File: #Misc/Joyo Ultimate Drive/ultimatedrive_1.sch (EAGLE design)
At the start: 36 parts, among them Q1 MSPA18, U2 JRC4558D, U3 NE5532N

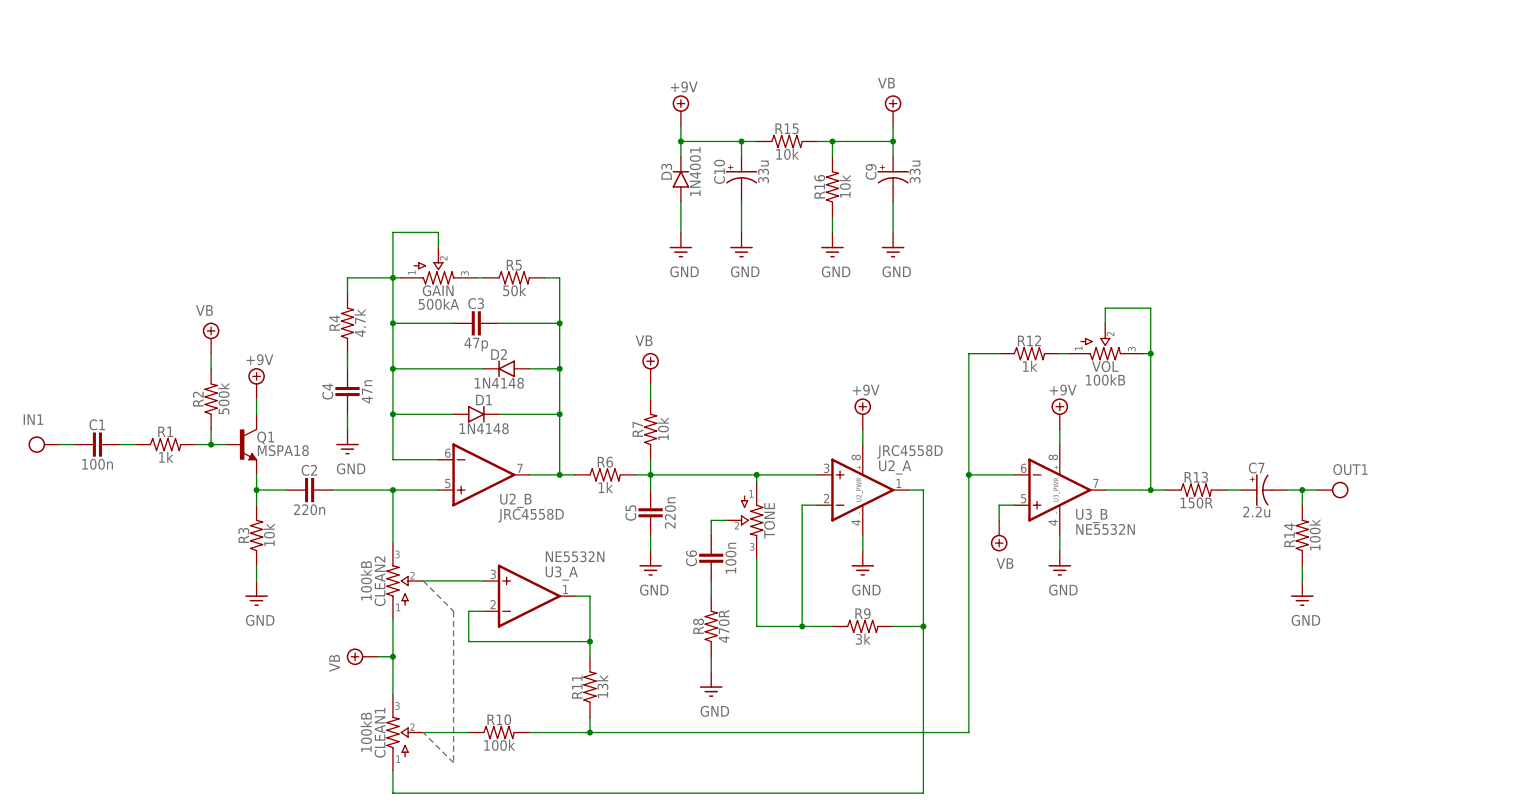
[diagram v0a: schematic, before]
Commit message: 20200320/09:17
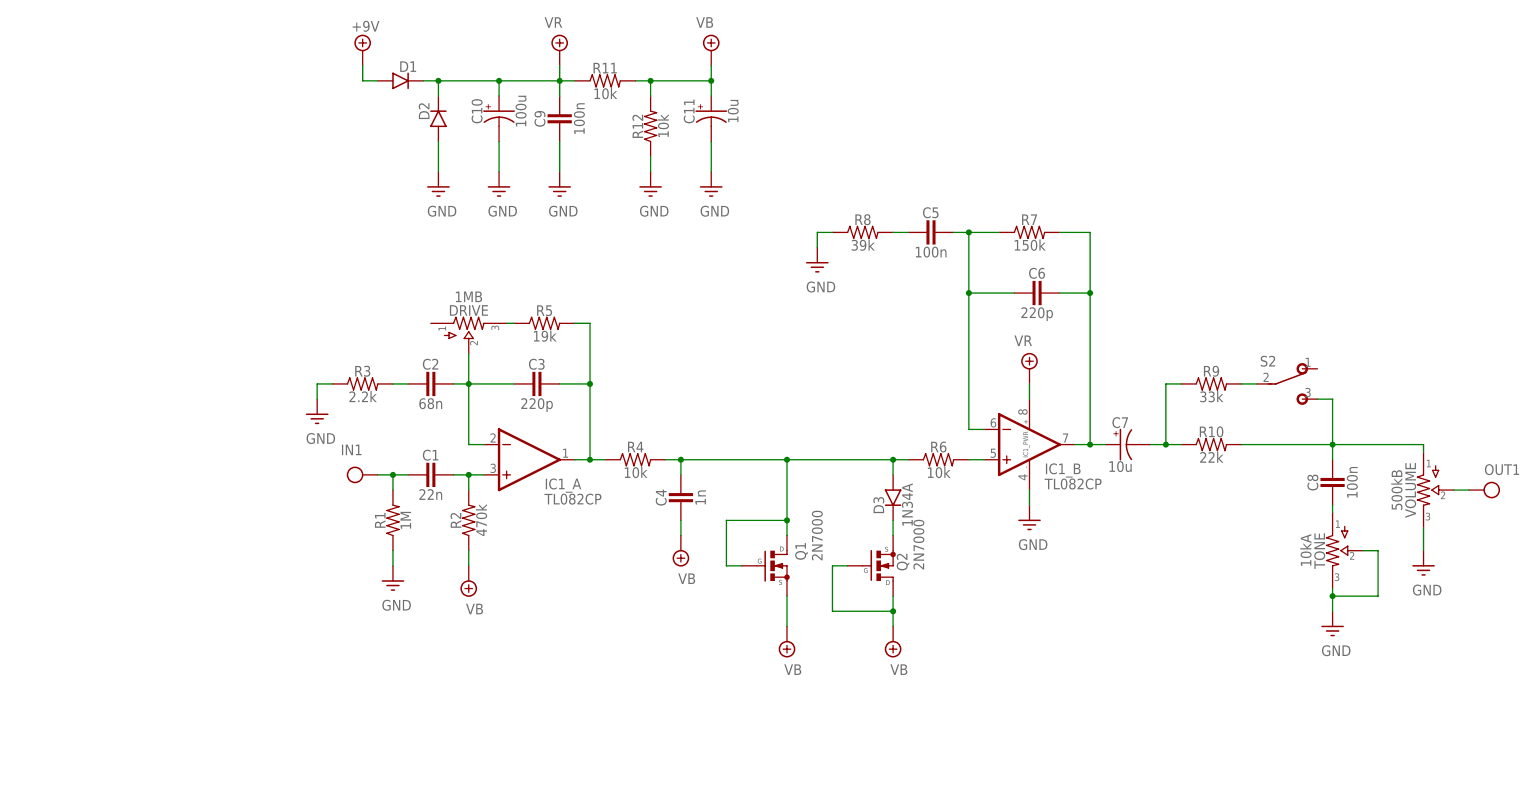
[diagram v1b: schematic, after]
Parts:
- removed CLEAN1, CLEAN2, VOL: 100kB, pedals-potentiometers:POTS16MM
- removed GAIN: 500kA, pedals-potentiometers:POTS16MM
- removed R13: 150R, pedals-resistors:R_.3B
- removed R14: 100k, pedals-resistors:R_.3B
- removed R15, R16: 10k, pedals-resistors:R_.3B
- removed U2: JRC4558D, pedals-integrated circuits:DUALTH
- removed U3: NE5532N, pedals-integrated circuits:DUALTH
- added C11: 10u, pedals-capacitors-elec:0500
- added C8: 100n, pedals-capacitors-film:CER/FILMBOX.1
- added DRIVE: 1MB, pedals-potentiometers:POTS16MM
- added IC1: TL082CP, pedals-integrated circuits:DUALTH
- added Q2: 2N7000, pedals-transistors:2N7000
- added S2: (no value), pedals-switches:SPDT
- added VOLUME: 500kB, pedals-potentiometers:POTS16MM
- C1: value 100n -> 22n
- C10: value 33u -> 100u
- C2: value 220n -> 68n
- C3: value 47p -> 220p
- C4: value 47n -> 1n
- C5: value 220n -> 100n
- C6: value 100n -> 220p
- C7: value 2.2u -> 10u
- C9: value 33u -> 100n; device pedals-capacitors-elec:0500 -> pedals-capacitors-film:CER/FILMBOX.1
- D1, D2: value 1N4148 -> (none); device pedals-diodes:DO35.2 -> pedals-diodes:DO41.3
- D3: value 1N4001 -> 1N34A; device pedals-diodes:DO35.3 -> pedals-diodes:DO41.2
- Q1: value MSPA18 -> 2N7000; device pedals-transistors:2N3904 -> pedals-transistors:2N7000
- R1: value 1k -> 1M
- R10: value 100k -> 22k
- R11: value 13k -> 10k
- R12, R6: value 1k -> 10k
- R2: value 500k -> 470k
- R3: value 10k -> 2.2k
- R4: value 4.7k -> 10k
- R5: value 50k -> 19k
- R7: value 10k -> 150k
- R8: value 470R -> 39k
- R9: value 3k -> 33k
- TONE: value (none) -> 10kA
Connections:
- removed net N$17: CLEAN1.1, R9.2, U2_A.OUT
- removed net N$18: CLEAN2.2, U3_A.+IN
- removed net N$19: C5.1, R6.2, R7.1, TONE.1, U2_A.+IN
- removed net N$21: C6.1, TONE.2
- removed net N$22: C6.2, R8.2
- removed net N$24: R12.2, VOL.1
- removed net N$25: R13.1, U3_B.OUT, VOL.2, VOL.3
- removed net N$28: C7.+, R13.2
- removed net N$3: GAIN.3, R5.1
- new net N$10: D3.C, Q2.S
- new net N$11: C4.1, D3.A, Q1.D, Q1.G, R4.2, R6.1
- new net N$16: C8.1, R10.2, S2.S, VOLUME.1
- new net N$7: C3.1, IC1_A.OUT, R4.1, R5.2
- new net VR: C10.+, C9.1, D1.C, D2.C, IC1_PWR.V+, R11.1
- net +9V: now also D1.A; no longer C10.+, D3.C, Q1.C, R15.1, U2_PWR.V+, U3_PWR.V+
- net GND: now also C11.-, C9.2, D2.A, IC1_PWR.V-, R1.1, R12.1, TONE.2, TONE.3, VOLUME.3; no longer C4.2, C5.2, C9.-, D3.A, R14.1, R16.1, U2_PWR.V-, U3_PWR.V-
- net IN: now also R1.2
- net N$1: now also C7.-, R10.1, R9.1; no longer C3.2, D1.A, D2.C, GAIN.1, GAIN.2, R4.2, U2_B.-IN
- net N$12: now also C5.1, C6.2, IC1_B.-IN, R7.1; no longer CLEAN1.2, R10.1
- net N$13: now also C6.1, C7.+, IC1_B.OUT, R7.2; no longer R11.2, U3_A.-IN, U3_A.OUT
- net N$14: now also C5.2, R8.2; no longer R9.1, TONE.3, U2_A.-IN
- net N$15: now also R9.2, S2.P; no longer R10.2, R11.1, R12.1, U3_B.-IN
- net N$2: now also C8.2, TONE.1; no longer C4.1, R4.1
- net N$4: now also C1.1, IC1_A.+IN, R2.2; no longer C3.1, D1.C, D2.A, R5.2, R6.1, U2_B.OUT
- net N$5: now also C3.2, DRIVE.2, IC1_A.-IN; no longer CLEAN2.3, U2_B.+IN
- net N$6: now also DRIVE.3, R5.1; no longer C2.2, Q1.E, R3.2
- net N$8: now also C2.2, R3.2; no longer C1.1, R1.1
- net N$9: now also IC1_B.+IN, R6.2; no longer Q1.B, R1.2, R2.1
- net OUT: now also VOLUME.2; no longer C7.-, R14.2
- net VB: now also C11.+, C4.2, Q1.S, Q2.D, Q2.G, R11.2, R12.2, R2.1; no longer C9.+, CLEAN1.3, CLEAN2.1, R15.2, R16.2, R2.2, R7.2, U3_B.+IN
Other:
- moved on the sheet: C1, C10, C2, C3, C4, C5, C6, C7, D1, D2, D3, R1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
